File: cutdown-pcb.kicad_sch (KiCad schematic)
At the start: 6 parts, among them J1 Conn_01x06

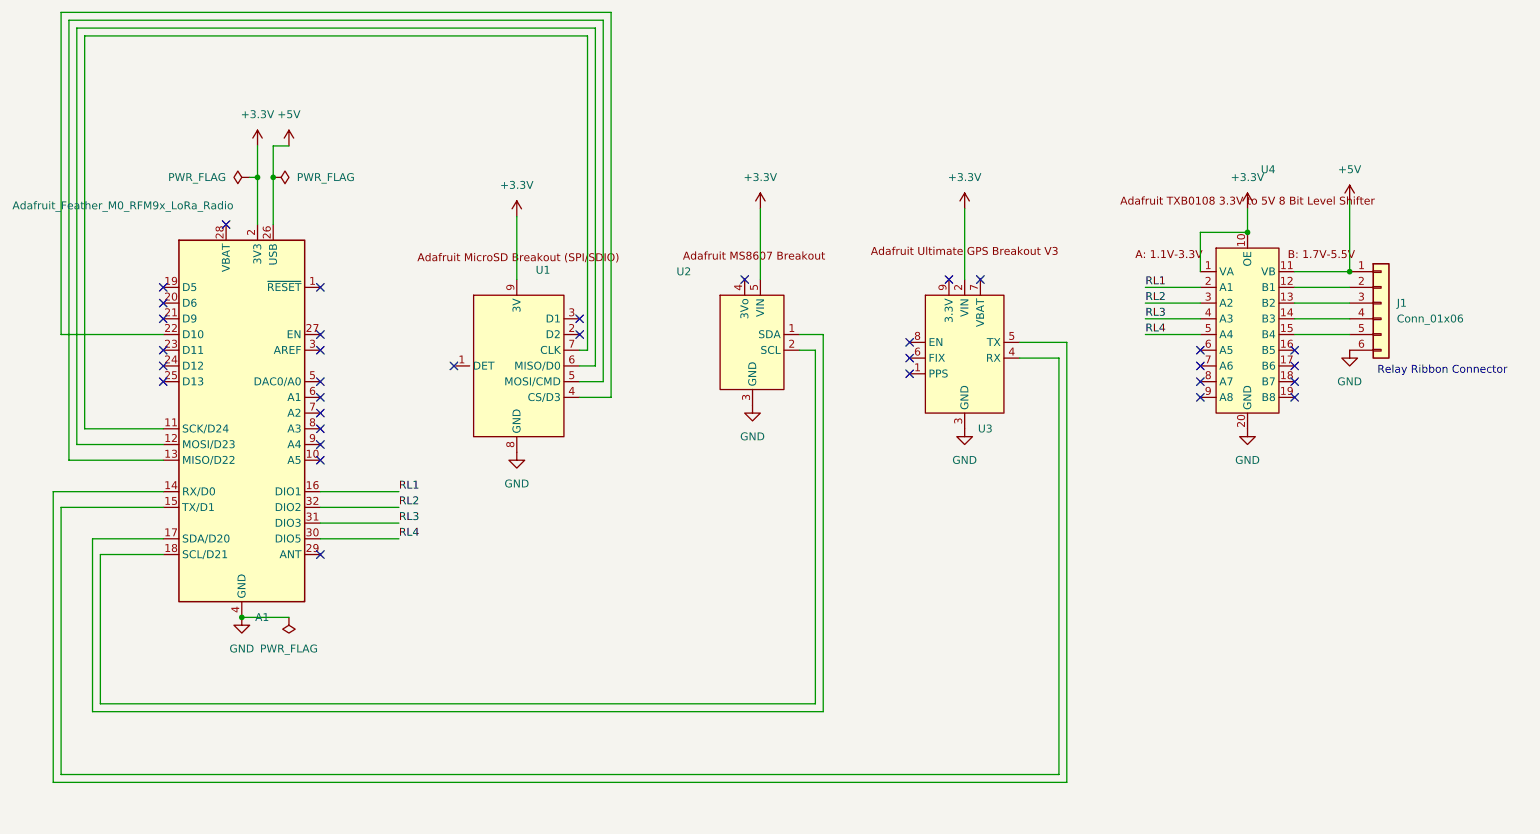
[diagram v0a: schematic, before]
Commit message: Version 3
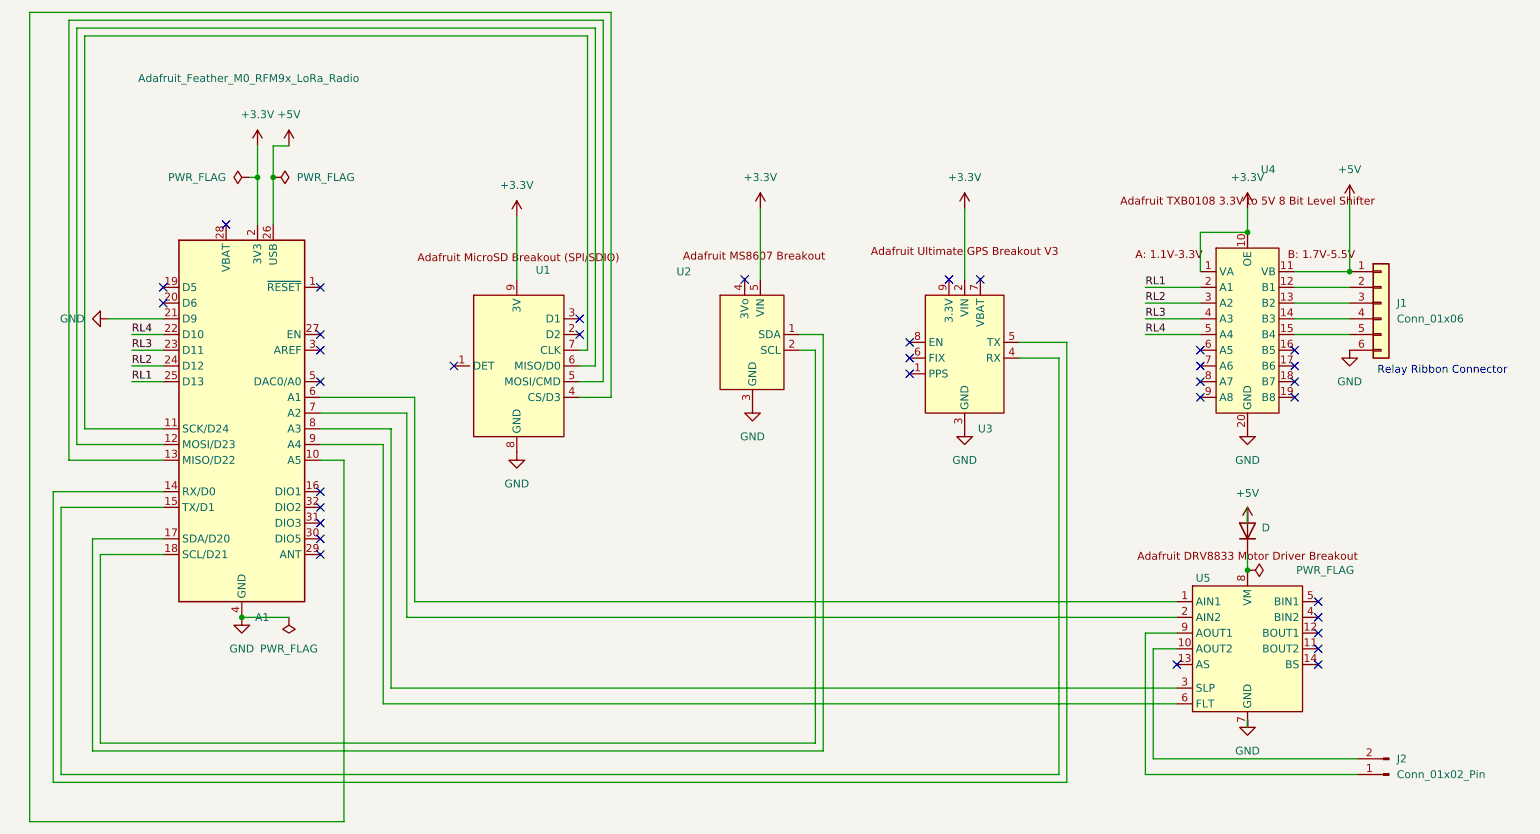
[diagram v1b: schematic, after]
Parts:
- added D1: D, Diode_THT:D_DO-35_SOD27_P10.16mm_Horizontal, symbol Device:D
- added J2: Conn_01x02_Pin, Connector_PinHeader_2.54mm:PinHeader_1x02_P2.54mm_Vertical, symbol Connector:Conn_01x02_Pin
- added U5: ~, CustomFootprints:AdafruitMotorDriverBreakout, symbol CustomSymbols:AdafruitDRV8833MotorDriverBreakout
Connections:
- net +5V: now also D1.2 (A)
- net GND: now also A1.21 (D9), U5.7 (GND)
- net RL1: now also A1.25 (D13); no longer A1.16 (DIO1)
- net RL2: now also A1.24 (D12); no longer A1.32 (DIO2)
- net RL3: now also A1.23 (D11); no longer A1.31 (DIO3)
- net RL4: now also A1.22 (D10); no longer A1.30 (DIO5)
- net at A1.10 (A5): now also U1.4 (CS/D3)
- net at A1.6 (A1): now also U5.1 (AIN1)
- net at A1.7 (A2): now also U5.2 (AIN2)
- net at A1.8 (A3): now also U5.3 (SLP)
- net at A1.9 (A4): now also U5.6 (FLT)
- new net: J2.2 (Pin_2), U5.10 (AOUT2)
- new net: D1.1 (K), U5.8 (VM)
- new net: J2.1 (Pin_1), U5.9 (AOUT1)
- no-connect marks 34 -> 35
